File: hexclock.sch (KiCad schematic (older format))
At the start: 39 parts, among them J1 USB_B_Micro, U1 ATtiny402-SS, U2 MCP7940N-xSN, Y1 7pF CL

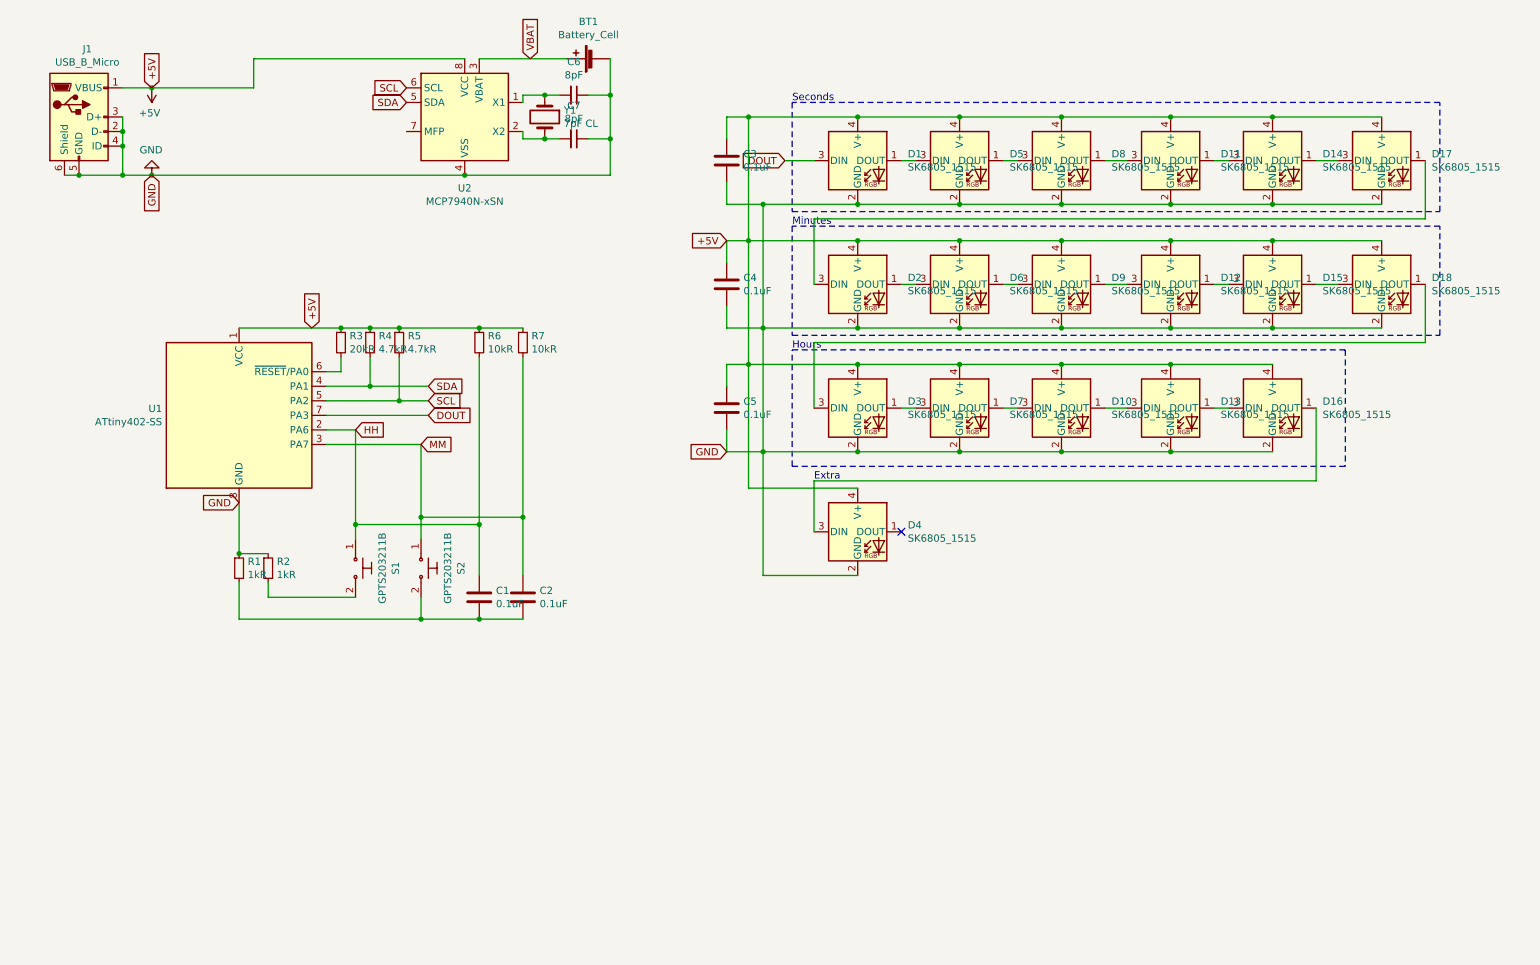
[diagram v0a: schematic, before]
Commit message: v0.0.0 finished
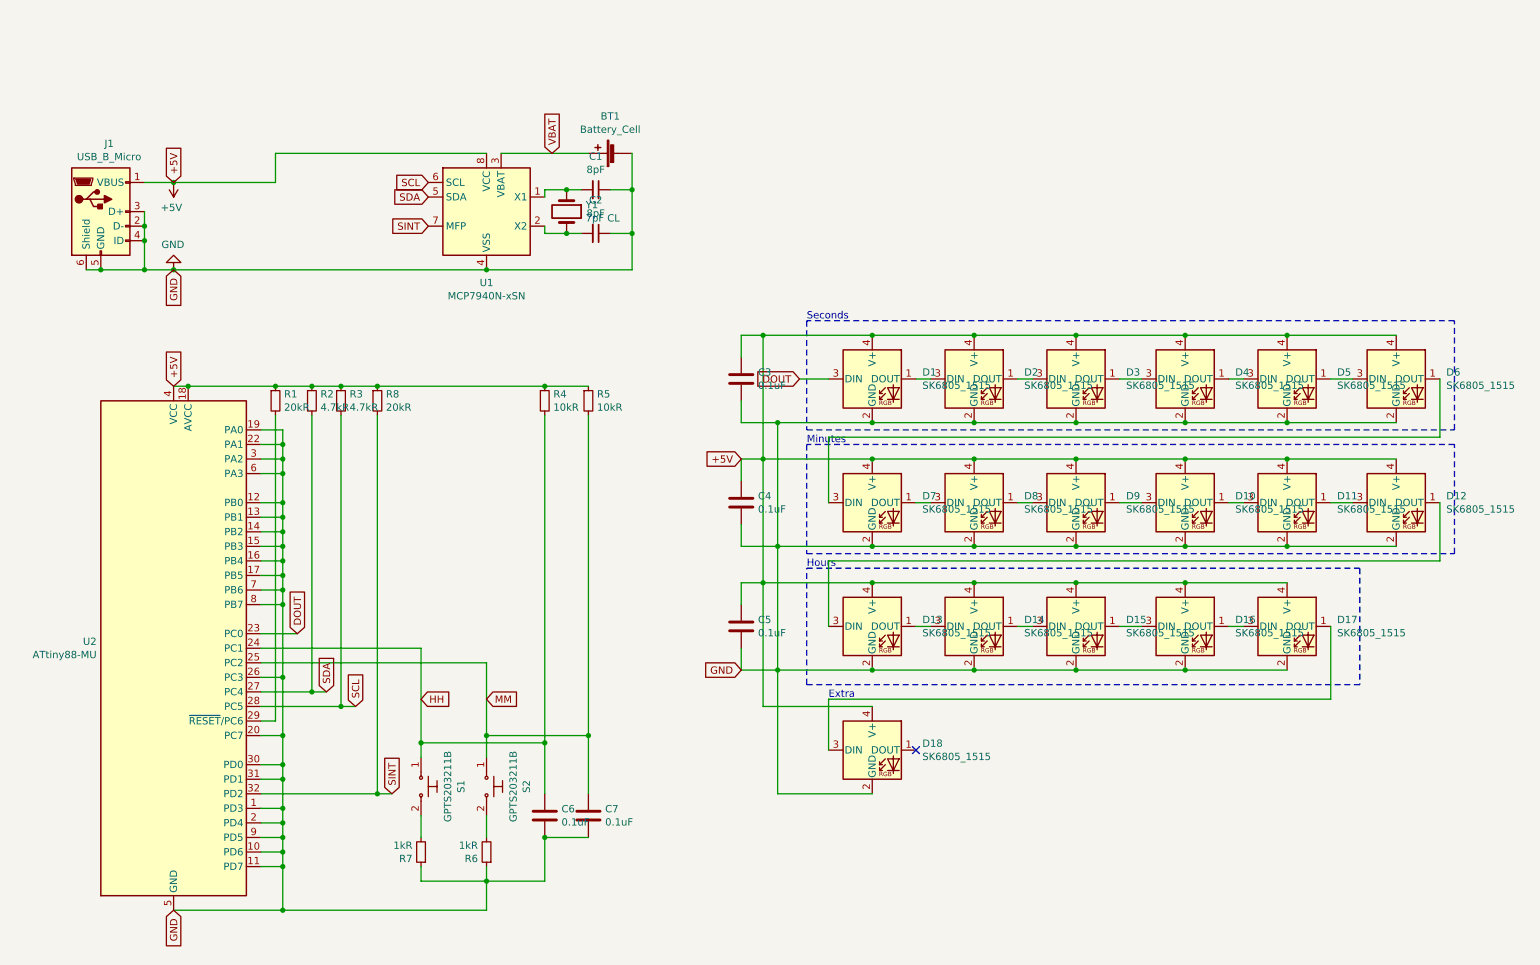
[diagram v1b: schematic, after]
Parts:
- removed U1: ATtiny402-SS, Package_SO:SOIC-8_3.9x4.9mm_P1.27mm, symbol MCU_Microchip_ATtiny:ATtiny402-SS
- added R8: 20kR, Resistor_SMD:R_0805_2012Metric, symbol Device:R_Small
- added U2: ATtiny88-MU, Package_DFN_QFN:QFN-32-1EP_5x5mm_P0.5mm_EP3.1x3.1mm, symbol MCU_Microchip_ATtiny:ATtiny88-MU
- U1: renamed from U2; footprint Package_SO:SOIC-8-1EP_3.9x4.9mm_P1.27mm_EP2.41x3.3mm -> Package_SO:SOIC-8_3.9x4.9mm_P1.27mm
- renumbered C6 to C1, C7 to C2, C1 to C6, C2 to C7, D12 to D10, D15 to D11, D18 to D12, D3 to D13, D7 to D14, D10 to D15, D13 to D16, D16 to D17, D4 to D18, D5 to D2, D8 to D3, D11 to D4, D14 to D5, D17 to D6, D2 to D7, D6 to D8, R3 to R1, R4 to R2, R5 to R3, R6 to R4, R7 to R5, R1 to R6, R2 to R7
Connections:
- net +5V: now also R8.1, U2.18 (AVCC), U2.4 (VCC)
- net DOUT: now also U2.23 (PC0)
- net GND: now also C6.2, C7.2, U2.1 (PD3), U2.10 (PD6), U2.11 (PD7), U2.12 (PB0), U2.13 (PB1), U2.14 (PB2), U2.15 (PB3), U2.16 (PB4), U2.17 (PB5), U2.19 (PA0), U2.2 (PD4), U2.20 (PC7), U2.21 (GND), U2.22 (PA1), U2.26 (PC3), U2.3 (PA2), U2.30 (PD0), U2.31 (PD1), U2.33 (GND), U2.5 (GND), U2.6 (PA3), U2.7 (PB6), U2.8 (PB7), U2.9 (PD5)
- net HH: now also U2.24 (PC1)
- net MM: now also U2.25 (PC2)
- net SCL: now also U2.28 (PC5)
- net SDA: now also U2.27 (PC4)
- net SINT: now reaches U1.7 (MFP)
- net SINT: now also R8.2, U2.32 (PD2)
- net at R6.2, S2.2: no longer C6.2, C7.2
- net at R1.2: now also U2.29 (~RESET~/PC6)
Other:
- moved on the sheet: BT1, C1, C2, C3, C4, C5, C6, C7, D1, D10, D11, D12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
